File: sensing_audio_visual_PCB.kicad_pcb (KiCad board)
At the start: 2 copper layers, 52 x 41.4 mm, 21 parts, among them J1 Amplifier, J10 220 ohm, J11 IR Emitter, J12 10k ohm, J13 IR Receiver, J14 220 ohm, J15 IR Emitter, J16 10k ohm, J17 IR Receiver, J18 220 ohm, J19 10k ohm, J2 OLED Display, J20 IR Emitter, J21 IR Receiver, J3 IR Emitter, J4 Light Strip, J5 Conn_01x03, J6 IR Receiver, J7 220 ohm, J8 10k ohm, J9 GPIO Pins

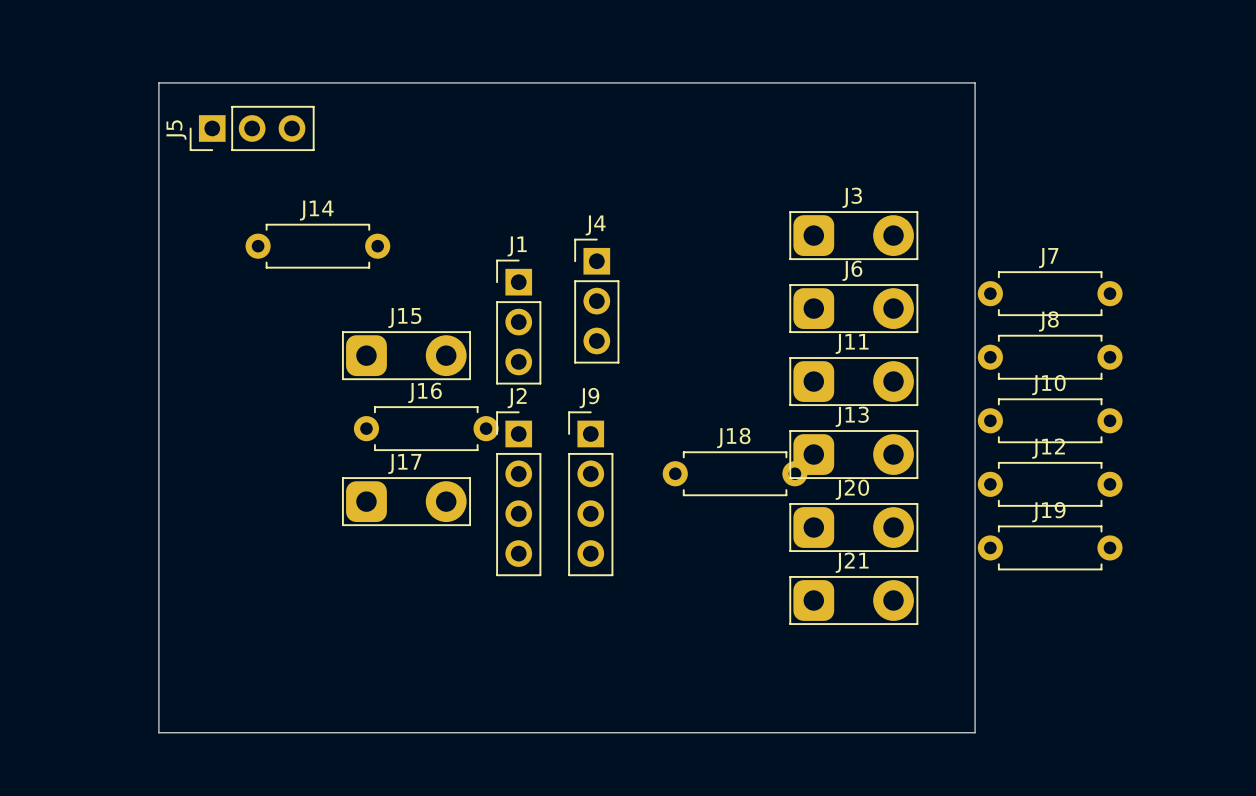
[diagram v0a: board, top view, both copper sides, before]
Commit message: Layout finished
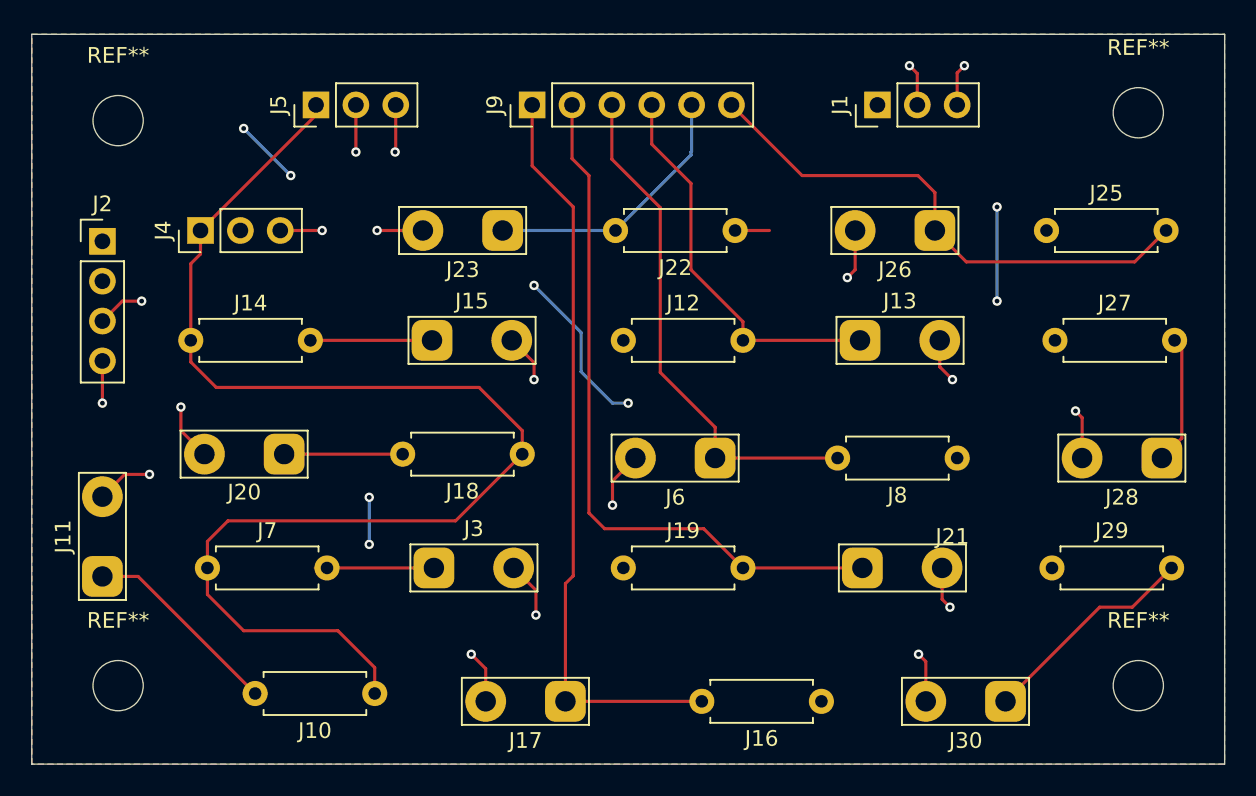
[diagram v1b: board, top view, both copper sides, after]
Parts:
- added J22: R_PhotoR, Resistor_THT:R_Axial_DIN0207_L6.3mm_D2.5mm_P7.62mm_Horizontal, F.Cu at (138.3, 74.0)
- added J23: photoresistor, TestPoint:TestPoint_2Pads_Pitch5.08mm_Drill1.3mm, F.Cu at (123.5, 74.0)
- added J25: R_PhotoR, Resistor_THT:R_Axial_DIN0207_L6.3mm_D2.5mm_P7.62mm_Horizontal, F.Cu at (158.2, 74.0)
- added J26: photoresistor, TestPoint:TestPoint_2Pads_Pitch5.08mm_Drill1.3mm, F.Cu at (151.0, 74.0)
- added J27: R_LED, Resistor_THT:R_Axial_DIN0207_L6.3mm_D2.5mm_P7.62mm_Horizontal, F.Cu at (158.7, 81.0)
- added J28: LED, TestPoint:TestPoint_2Pads_Pitch5.08mm_Drill1.3mm, F.Cu at (165.5, 88.5)
- added J29: R_LED, Resistor_THT:R_Axial_DIN0207_L6.3mm_D2.5mm_P7.62mm_Horizontal, F.Cu at (158.5, 95.5)
- added J30: LED, TestPoint:TestPoint_2Pads_Pitch5.08mm_Drill1.3mm, F.Cu at (155.5, 104.0)
- added REF**: MountingHole_3.2mm_M3, MountingHole:MountingHole_3.2mm_M3, F.Cu at (99.0, 67.0)
- added REF**: MountingHole_3.2mm_M3, MountingHole:MountingHole_3.2mm_M3, F.Cu at (164.0, 103.0)
- added REF**: MountingHole_3.2mm_M3, MountingHole:MountingHole_3.2mm_M3, F.Cu at (99.0, 103.0)
- added REF**: MountingHole_3.2mm_M3, MountingHole:MountingHole_3.2mm_M3, F.Cu at (164.0, 66.5)
- J10, J14, J18, J7: value 220 ohm -> R_emitter
- J12, J16, J19, J8: value 10k ohm -> R_receiver
- J9: value GPIO Pins -> Conn_01x06; footprint Connector_PinHeader_2.54mm:PinHeader_1x04_P2.54mm_Vertical -> Connector_PinHeader_2.54mm:PinHeader_1x06_P2.54mm_Vertical
- moved J7 52.9 mm to (104.7, 95.5)
- moved J11 47.0 mm to (98.0, 96.0), turned to 90 degrees
- moved J10 42.9 mm to (115.3, 103.5), turned to 180 degrees
- moved J20 34.1 mm to (109.6, 88.2), turned to 180 degrees
- moved J16 33.8 mm to (143.8, 104.0), turned to 180 degrees
- moved J3 32.2 mm to (119.1, 95.5)
- moved J2 29.2 mm to (98.0, 74.7)
- moved J1 25.5 mm to (147.4, 66.0), turned to 90 degrees
- moved J4 25.3 mm to (104.2, 74.0), turned to 90 degrees
- moved J12 25.1 mm to (131.2, 81.0)
- moved J19 23.4 mm to (131.2, 95.5)
- moved J9 21.3 mm to (125.4, 66.0), turned to 90 degrees
- moved J17 18.0 mm to (127.5, 104.0), turned to 180 degrees
- moved J6 11.4 mm to (137.0, 88.5), turned to 180 degrees
- moved J18 9.83 mm to (124.8, 88.2), turned to 180 degrees
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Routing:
- net /5V: track 0.00 -> 84.4 mm
- net /GND: track 0.00 -> 50.0 mm, vias 0 -> 16
- net Net-(J16-Pin_2): track 0.00 -> 47.5 mm
- net Net-(J19-Pin_2): track 0.00 -> 44.8 mm
- net /3V3: track 0.00 -> 35.0 mm, vias 0 -> 11
- net Net-(J25-Pin_2): track 0.00 -> 34.1 mm
- net Net-(J6-Pin_1): track 0.00 -> 32.5 mm
- net Net-(J12-Pin_2): track 0.00 -> 24.9 mm
- net Net-(J22-Pin_2): track 0.00 -> 17.2 mm
- net Net-(J29-Pin_2): track 0.00 -> 14.1 mm
- net Net-(J10-Pin_2): track 0.00 -> 12.8 mm
- net Net-(J27-Pin_2): track 0.00 -> 8.03 mm
- net Net-(J18-Pin_2): track 0.00 -> 7.55 mm
- net Net-(J14-Pin_2): track 0.00 -> 6.75 mm
- net Net-(J3-Pin_1): track 0.00 -> 6.56 mm
- added copper zone on F.Cu, net /3V3
- added copper zone on B.Cu, net /GND
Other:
- board size 52 x 41.4 mm -> 76 x 46.5 mm
